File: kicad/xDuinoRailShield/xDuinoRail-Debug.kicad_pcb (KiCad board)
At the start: 2 copper layers, 99.7 x 99.7 mm, 68 parts, among them J201 USB_B, J202 SWCLK, J203 SWDIO, J204 RUN, J301 21mtc_mrkl, J401 Conn_01x06, J601 Screw_Terminal_01x02, J701 Screw_Terminal_01x02, J801 Screw_Terminal_01x02, Q901 BC847BVN, Q902 BC847BVN, U201 RP2040, U501 LM339, Y201 X322512MSB4SI

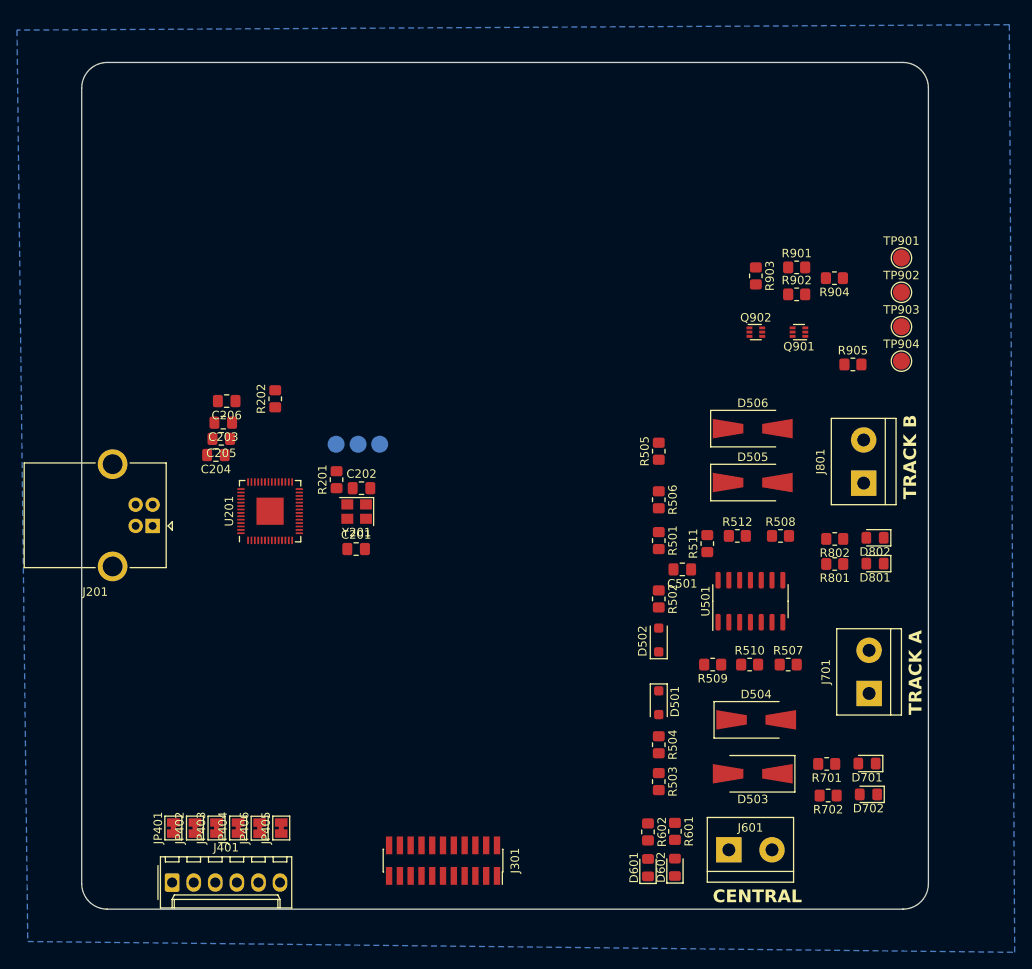
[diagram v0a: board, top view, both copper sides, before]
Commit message: More stuff
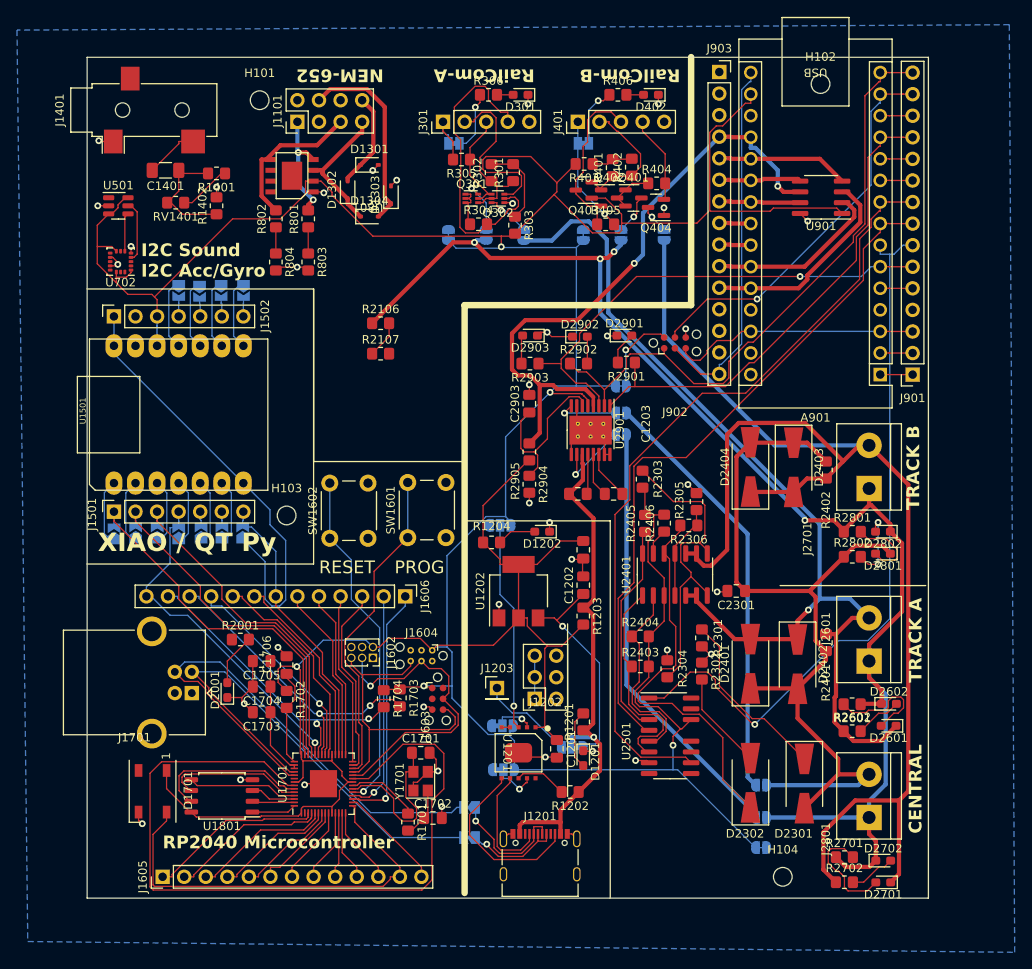
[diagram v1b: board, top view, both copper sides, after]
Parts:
- removed C201, C202: 33p, Capacitor_SMD:C_0805_2012Metric_Pad1.18x1.45mm_HandSolder
- removed C203, C204: 100n, Capacitor_SMD:C_0805_2012Metric_Pad1.18x1.45mm_HandSolder
- removed C205, C206: 10u, Capacitor_SMD:C_0805_2012Metric_Pad1.18x1.45mm_HandSolder
- removed C501: 47uF, Capacitor_SMD:C_0805_2012Metric_Pad1.18x1.45mm_HandSolder
- removed D501, D502: 1N4004, Diode_SMD:D_SOD-123F
- removed D503, D504, D505, D506: SS54, Diode_SMD:D_SMA-SMB_Universal_Handsoldering
- removed D601, D602, D701, D702, D801, D802: LED, LED_SMD:LED_0805_2012Metric_Pad1.15x1.40mm_HandSolder
- removed J202: SWCLK, TestPoint:TestPoint_Pad_D2.0mm
- removed J203: SWDIO, TestPoint:TestPoint_Pad_D2.0mm
- removed J204: RUN, TestPoint:TestPoint_Pad_D2.0mm
- removed J601, J701, J801: Screw_Terminal_01x02, TerminalBlock:TerminalBlock_bornier-2_P5.08mm
- removed JP402, JP403, JP404, JP405, JP406: SolderJumper_2_Bridged, Jumper:SolderJumper-2_P1.3mm_Bridged_Pad1.0x1.5mm
- removed Q901, Q902: BC847BVN, Package_TO_SOT_SMD:SOT-563
- removed R201: 1k, Resistor_SMD:R_0805_2012Metric_Pad1.20x1.40mm_HandSolder
- removed R202: 200R, Resistor_SMD:R_0805_2012Metric_Pad1.20x1.40mm_HandSolder
- removed R501, R502: 220R, Resistor_SMD:R_0805_2012Metric_Pad1.20x1.40mm_HandSolder
- removed R503: 270K, Resistor_SMD:R_0805_2012Metric_Pad1.20x1.40mm_HandSolder
- removed R504: 1K, Resistor_SMD:R_0805_2012Metric_Pad1.20x1.40mm_HandSolder
- removed R505: 820R, Resistor_SMD:R_0805_2012Metric_Pad1.20x1.40mm_HandSolder
- removed R506: 33k, Resistor_SMD:R_0805_2012Metric_Pad1.20x1.40mm_HandSolder
- removed R507, R508: 1R8, Resistor_SMD:R_0805_2012Metric_Pad1.20x1.40mm_HandSolder
- removed R509, R510, R511, R512: 10K, Resistor_SMD:R_0805_2012Metric_Pad1.20x1.40mm_HandSolder
- removed R601, R602, R701, R702: 3k3, Resistor_SMD:R_0805_2012Metric_Pad1.20x1.40mm_HandSolder
- removed R901, R902, R903: 10R, Resistor_SMD:R_0805_2012Metric_Pad1.20x1.40mm_HandSolder
- removed R904, R905: 10k, Resistor_SMD:R_0805_2012Metric_Pad1.20x1.40mm_HandSolder
- removed TP901, TP902, TP903, TP904: TestPoint, TestPoint:TestPoint_Pad_D2.0mm
- removed U201: RP2040, Package_DFN_QFN:QFN-56-1EP_7x7mm_P0.4mm_EP3.2x3.2mm
- removed Y201: X322512MSB4SI, Crystal:Crystal_SMD_3225-4Pin_3.2x2.5mm
- added A901: Arduino_Nano_Every, Module:Arduino_Nano, F.Cu at (177.2, 72.9)
- added C1201: 1uF, Capacitor_SMD:C_0805_2012Metric_Pad1.18x1.45mm_HandSolder, F.Cu at (139.1, 117.0)
- added C1202: 1uF, Capacitor_SMD:C_0805_2012Metric_Pad1.18x1.45mm_HandSolder, F.Cu at (142.2, 97.7)
- added C1203: 47uF, Capacitor_SMD:C_0805_2012Metric_Pad1.18x1.45mm_HandSolder, F.Cu at (142.2, 93.6)
- added C1401: 100uF, Capacitor_SMD:C_1206_3216Metric_Pad1.33x1.80mm_HandSolder, F.Cu at (93.1, 48.9)
- added C1701: 33p, Capacitor_SMD:C_0805_2012Metric_Pad1.18x1.45mm_HandSolder, F.Cu at (123.1, 117.5)
- added C1702: 33p, Capacitor_SMD:C_0805_2012Metric_Pad1.18x1.45mm_HandSolder, F.Cu at (124.5, 125.2)
- added C1703: 100n, Capacitor_SMD:C_0805_2012Metric_Pad1.18x1.45mm_HandSolder, F.Cu at (104.4, 112.7)
- added C1704: 100n, Capacitor_SMD:C_0805_2012Metric_Pad1.18x1.45mm_HandSolder, F.Cu at (104.4, 109.7)
- added C1705: 10u, Capacitor_SMD:C_0805_2012Metric_Pad1.18x1.45mm_HandSolder, F.Cu at (104.4, 106.7)
- added C1706: 10u, Capacitor_SMD:C_0805_2012Metric_Pad1.18x1.45mm_HandSolder, F.Cu at (107.3, 107.2)
- added C2301: 47uF, Capacitor_SMD:C_0805_2012Metric_Pad1.18x1.45mm_HandSolder, F.Cu at (160.3, 98.4)
- added C2901: 100nF, Capacitor_SMD:C_0805_2012Metric_Pad1.18x1.45mm_HandSolder, F.Cu at (141.6, 87.0)
- added C2902: 22nF, Capacitor_SMD:C_0805_2012Metric_Pad1.18x1.45mm_HandSolder, F.Cu at (145.8, 87.0)
- added C2903: 22nF, Capacitor_SMD:C_0805_2012Metric_Pad1.18x1.45mm_HandSolder, F.Cu at (135.9, 76.4)
- added D1201: LED, LED_SMD:LED_0603_1608Metric_Pad1.05x0.95mm_HandSolder, F.Cu at (142.2, 118.1)
- added D1202: LED, LED_SMD:LED_0603_1608Metric_Pad1.05x0.95mm_HandSolder, F.Cu at (137.4, 91.4)
- added D1301: 1N5819WS, Diode_SMD:D_SOD-323, F.Cu at (117.1, 48.3)
- added D1302: 1N5819WS, Diode_SMD:D_SOD-323, F.Cu at (114.5, 51.2)
- added D1303: 1N5819WS, Diode_SMD:D_SOD-323, F.Cu at (119.6, 51.8)
- added D1304: 1N5819WS, Diode_SMD:D_SOD-323, F.Cu at (117.1, 54.3)
- added D1701: WS2812B, LED_SMD:LED_WS2812B_PLCC4_5.0x5.0mm_P3.2mm, F.Cu at (91.5, 122.0)
- added D2001: LED, LED_SMD:LED_0603_1608Metric_Pad1.05x0.95mm_HandSolder, F.Cu at (100.3, 110.1)
- added D2301: SM4007, Diode_SMD:D_SMA-SMB_Universal_Handsoldering, F.Cu at (168.3, 121.1)
- added D2302: SM4007, Diode_SMD:D_SMA-SMB_Universal_Handsoldering, F.Cu at (161.9, 121.0)
- added D2401: SS54, Diode_SMD:D_SMA-SMB_Universal_Handsoldering, F.Cu at (161.9, 107.0)
- added D2402: SS54, Diode_SMD:D_SMA-SMB_Universal_Handsoldering, F.Cu at (167.5, 107.0)
- added D2403: SS54, Diode_SMD:D_SMA-SMB_Universal_Handsoldering, F.Cu at (167.0, 83.9)
- added D2404: SS54, Diode_SMD:D_SMA-SMB_Universal_Handsoldering, F.Cu at (161.9, 83.8)
- added D2601: LED, LED_SMD:LED_0603_1608Metric_Pad1.05x0.95mm_HandSolder, F.Cu at (178.2, 114.3)
- added D2602: LED, LED_SMD:LED_0603_1608Metric_Pad1.05x0.95mm_HandSolder, F.Cu at (178.2, 111.7)
- added D2701: LED, LED_SMD:LED_0603_1608Metric_Pad1.05x0.95mm_HandSolder, F.Cu at (177.6, 132.7)
- added D2702: LED, LED_SMD:LED_0603_1608Metric_Pad1.05x0.95mm_HandSolder, F.Cu at (177.6, 130.2)
- added D2801: LED, LED_SMD:LED_0603_1608Metric_Pad1.05x0.95mm_HandSolder, F.Cu at (177.5, 94.0)
- added D2802: LED, LED_SMD:LED_0603_1608Metric_Pad1.05x0.95mm_HandSolder, F.Cu at (177.5, 91.4)
- added D2901: LED_RED, LED_SMD:LED_0603_1608Metric_Pad1.05x0.95mm_HandSolder, F.Cu at (147.1, 68.3)
- added D2902: LED_YELLOW, LED_SMD:LED_0603_1608Metric_Pad1.05x0.95mm_HandSolder, F.Cu at (141.8, 68.5)
- added D2903: LED_GREEN, LED_SMD:LED_0603_1608Metric_Pad1.05x0.95mm_HandSolder, F.Cu at (136.0, 68.3)
- added D301: LED, LED_SMD:LED_0603_1608Metric_Pad1.05x0.95mm_HandSolder, F.Cu at (134.9, 40.0)
- added D402: LED, LED_SMD:LED_0603_1608Metric_Pad1.05x0.95mm_HandSolder, F.Cu at (150.2, 40.0)
- added H101: MountingHole, MountingHole:MountingHole_2.2mm_M2, F.Cu at (104.1, 40.6)
- added H102: MountingHole, MountingHole:MountingHole_2.2mm_M2, F.Cu at (170.2, 38.7)
- added H103: MountingHole, MountingHole:MountingHole_2.2mm_M2, F.Cu at (107.3, 89.5)
- added H104: MountingHole, MountingHole:MountingHole_2.2mm_M2, F.Cu at (165.7, 132.1)
- added J1101: Conn_02x04_Counter_Clockwise, Connector_PinHeader_2.54mm:PinHeader_2x04_P2.54mm_Vertical, F.Cu at (108.6, 43.2)
- added J1201: USB_C_Receptacle_USB2.0_14P, Connector_USB:USB_C_Receptacle_Palconn_UTC16-G, F.Cu at (137.2, 129.5)
- added J1202: Conn_02x03_Odd_Even, Connector_PinSocket_2.54mm:PinSocket_2x03_P2.54mm_Vertical, F.Cu at (136.5, 111.1)
- added J1203: Conn_01x01, Connector_PinHeader_2.54mm:PinHeader_1x01_P2.54mm_Vertical, F.Cu at (132.1, 109.9)
- added J1401: AudioJack2_Ground, Connector_Audio:Jack_3.5mm_CUI_SJ-3523-SMT_Horizontal, F.Cu at (90.5, 41.8)
- added J1501: Conn_01x07, Connector_PinSocket_2.54mm:PinSocket_1x07_P2.54mm_Vertical, F.Cu at (87.0, 89.1)
- added J1502: Conn_01x07, Connector_PinSocket_2.54mm:PinSocket_1x07_P2.54mm_Vertical, F.Cu at (87.0, 66.1)
- added J1602: Conn_02x03_Odd_Even, Connector_PinSocket_1.27mm:PinSocket_2x03_P1.27mm_Vertical, F.Cu at (117.5, 106.3)
- added J1603: Conn_ARM_SWD_TagConnect_TC2030-NL, Connector:Tag-Connect_TC2030-IDC-NL_2x03_P1.27mm_Vertical, F.Cu at (125.1, 111.1)
- added J1604: Conn_ARM_SWD_TagConnect_TC2030-NL, xDuinoRailShield:Tag-Connect_TC2030-IDC-NL_2x03_P1.27mm_Vertical-WithHoles, F.Cu at (123.2, 106.0)
- added J1605: Conn_01x13, Connector_PinHeader_2.54mm:PinHeader_1x13_P2.54mm_Vertical, F.Cu at (92.7, 132.1)
- added J1606: Conn_01x13, Connector_PinHeader_2.54mm:PinHeader_1x13_P2.54mm_Vertical, F.Cu at (121.3, 99.1)
- added J2601: Screw_Terminal_01x02, TerminalBlock:TerminalBlock_bornier-2_P5.08mm, F.Cu at (175.9, 106.7)
- added J2701: Screw_Terminal_01x02, TerminalBlock:TerminalBlock_bornier-2_P5.08mm, F.Cu at (175.9, 86.4)
- added J2801: Screw_Terminal_01x02, TerminalBlock:TerminalBlock_bornier-2_P5.08mm, F.Cu at (175.9, 125.1)
- added J901: Conn_01x15, Connector_PinSocket_2.54mm:PinSocket_1x15_P2.54mm_Vertical, F.Cu at (181.0, 73.0)
- added J902: Conn_ARM_SWD_TagConnect_TC2030-NL, Connector:Tag-Connect_TC2030-IDC-NL_2x03_P1.27mm_Vertical, F.Cu at (153.0, 69.2)
- added J903: Conn_01x15, Connector_PinSocket_2.54mm:PinSocket_1x15_P2.54mm_Vertical, F.Cu at (158.3, 37.3)
- added JP1001: SolderJumper_2_Open, Jumper:SolderJumper-2_P1.3mm_Open_RoundedPad1.0x1.5mm, B.Cu at (146.7, 77.5)
- added JP1002: SolderJumper_2_Open, Jumper:SolderJumper-2_P1.3mm_Open_RoundedPad1.0x1.5mm, B.Cu at (146.7, 80.0)
- added JP1003: SolderJumper_2_Open, Jumper:SolderJumper-2_P1.3mm_Open_RoundedPad1.0x1.5mm, B.Cu at (146.7, 74.3)
- added JP1201: CFG2, Jumper:SolderJumper-3_P1.3mm_Bridged12_RoundedPad1.0x1.5mm_NumberLabels, B.Cu at (132.7, 114.3)
- added JP1202: CFG3, Jumper:SolderJumper-3_P1.3mm_Bridged12_RoundedPad1.0x1.5mm_NumberLabels, B.Cu at (132.4, 90.7)
- added JP1203: CFG1, Jumper:SolderJumper-3_P1.3mm_Bridged12_RoundedPad1.0x1.5mm_NumberLabels, B.Cu at (132.8, 119.5)
- added JP1204: CFG1, Jumper:SolderJumper-3_P1.3mm_Bridged12_RoundedPad1.0x1.5mm_NumberLabels, B.Cu at (140.9, 116.8)
- added JP1205: SolderJumper_2_Open, Jumper:SolderJumper-2_P1.3mm_Open_TrianglePad1.0x1.5mm, B.Cu at (128.8, 123.9)
- added JP1206: SolderJumper_2_Open, Jumper:SolderJumper-2_P1.3mm_Open_TrianglePad1.0x1.5mm, B.Cu at (128.8, 127.5)
- added JP1501: SolderJumper_2_Open, Jumper:SolderJumper-2_P1.3mm_Open_TrianglePad1.0x1.5mm, B.Cu at (87.0, 91.7)
- added JP1502: SolderJumper_2_Open, Jumper:SolderJumper-2_P1.3mm_Open_TrianglePad1.0x1.5mm, B.Cu at (92.1, 91.6)
- added JP1503: SolderJumper_2_Open, Jumper:SolderJumper-2_P1.3mm_Open_TrianglePad1.0x1.5mm, B.Cu at (89.5, 91.6)
- added JP1504: SolderJumper_2_Open, Jumper:SolderJumper-2_P1.3mm_Open_TrianglePad1.0x1.5mm, B.Cu at (94.6, 91.7)
- added JP1505: SolderJumper_2_Open, Jumper:SolderJumper-2_P1.3mm_Open_TrianglePad1.0x1.5mm, B.Cu at (97.2, 91.6)
- added JP1506: SolderJumper_2_Open, Jumper:SolderJumper-2_P1.3mm_Open_TrianglePad1.0x1.5mm, B.Cu at (99.7, 91.6)
- added JP1507: SolderJumper_2_Open, Jumper:SolderJumper-2_P1.3mm_Open_TrianglePad1.0x1.5mm, B.Cu at (102.1, 91.6)
- added JP1508: SolderJumper_2_Open, Jumper:SolderJumper-2_P1.3mm_Open_TrianglePad1.0x1.5mm, B.Cu at (102.2, 63.0)
- added JP1509: SolderJumper_2_Open, Jumper:SolderJumper-2_P1.3mm_Open_TrianglePad1.0x1.5mm, B.Cu at (99.6, 63.0)
- added JP1510: SolderJumper_2_Open, Jumper:SolderJumper-2_P1.3mm_Open_TrianglePad1.0x1.5mm, B.Cu at (97.1, 63.1)
- added JP1511: SolderJumper_2_Open, Jumper:SolderJumper-2_P1.3mm_Open_TrianglePad1.0x1.5mm, B.Cu at (94.6, 63.0)
- added JP1901: SolderJumper_2_Open, Jumper:SolderJumper-2_P1.3mm_Open_RoundedPad1.0x1.5mm, B.Cu at (135.3, 56.5)
- added JP1902: SolderJumper_2_Open, Jumper:SolderJumper-2_P1.3mm_Open_RoundedPad1.0x1.5mm, B.Cu at (130.8, 56.5)
- added JP1903: SolderJumper_2_Open, Jumper:SolderJumper-2_P1.3mm_Open_RoundedPad1.0x1.5mm, B.Cu at (126.4, 56.5)
- added JP201: SolderJumper_2_Open, Jumper:SolderJumper-2_P1.3mm_Open_RoundedPad1.0x1.5mm, B.Cu at (151.8, 56.5)
- added JP202: SolderJumper_2_Open, Jumper:SolderJumper-2_P1.3mm_Open_RoundedPad1.0x1.5mm, B.Cu at (146.7, 56.5)
- added JP203: SolderJumper_2_Open, Jumper:SolderJumper-2_P1.3mm_Open_RoundedPad1.0x1.5mm, B.Cu at (142.2, 56.5)
- added JP301: SolderJumper_2_Bridged, Jumper:SolderJumper-2_P1.3mm_Bridged_Pad1.0x1.5mm, B.Cu at (127.0, 45.7)
- added JP601: SolderJumper_2_Open, Jumper:SolderJumper-2_P1.3mm_Open_RoundedPad1.0x1.5mm, B.Cu at (163.2, 121.3)
- added JP602: SolderJumper_2_Open, Jumper:SolderJumper-2_P1.3mm_Open_RoundedPad1.0x1.5mm, B.Cu at (163.2, 125.1)
- added JP603: SolderJumper_2_Open, Jumper:SolderJumper-2_P1.3mm_Open_RoundedPad1.0x1.5mm, B.Cu at (163.2, 128.6)
- added Q301: BC847BVN, Package_TO_SOT_SMD:SOT-563, F.Cu at (129.1, 52.2)
- added Q302: BC847BVN, Package_TO_SOT_SMD:SOT-563, F.Cu at (132.2, 52.2)
- added Q401: S8050, Package_TO_SOT_SMD:SOT-23, F.Cu at (148.1, 52.2)
- added Q402: S8550, Package_TO_SOT_SMD:SOT-23, F.Cu at (145.3, 52.2)
- added Q403: S8550, Package_TO_SOT_SMD:SOT-23, F.Cu at (142.3, 51.2)
- added Q404: S8050, Package_TO_SOT_SMD:SOT-23, F.Cu at (150.8, 53.3)
- added R1201: 1k, Resistor_SMD:R_0805_2012Metric_Pad1.20x1.40mm_HandSolder, F.Cu at (142.2, 113.8)
- added R1202: 10k, Resistor_SMD:R_0805_2012Metric_Pad1.20x1.40mm_HandSolder, F.Cu at (140.7, 122.1)
- added R1203: 1k, Resistor_SMD:R_0805_2012Metric_Pad1.20x1.40mm_HandSolder, F.Cu at (142.2, 101.4)
- added R1204: 100R, Resistor_SMD:R_0805_2012Metric_Pad1.20x1.40mm_HandSolder, F.Cu at (131.4, 92.7)
- added R1401: 10k, Resistor_SMD:R_0805_2012Metric_Pad1.20x1.40mm_HandSolder, F.Cu at (99.1, 49.3)
- added R1402: 10k, Resistor_SMD:R_0805_2012Metric_Pad1.20x1.40mm_HandSolder, F.Cu at (99.1, 53.1)
- added R1701: 1k, Resistor_SMD:R_0805_2012Metric_Pad1.20x1.40mm_HandSolder, F.Cu at (121.6, 125.6)
- added R1702: 220R, Resistor_SMD:R_0805_2012Metric_Pad1.20x1.40mm_HandSolder, F.Cu at (107.3, 111.2)
- added R1703: 10k, Resistor_SMD:R_0805_2012Metric_Pad1.20x1.40mm_HandSolder, F.Cu at (120.7, 111.0)
- added R1704: 10k, Resistor_SMD:R_0805_2012Metric_Pad1.20x1.40mm_HandSolder, F.Cu at (118.7, 111.1)
- added R2001: 470R, Resistor_SMD:R_0805_2012Metric_Pad1.20x1.40mm_HandSolder, F.Cu at (101.9, 104.1)
- added R2106: 10k, Resistor_SMD:R_0805_2012Metric_Pad1.20x1.40mm_HandSolder, F.Cu at (118.4, 66.9)
- added R2107: 10k, Resistor_SMD:R_0805_2012Metric_Pad1.20x1.40mm_HandSolder, F.Cu at (118.4, 70.5)
- added R2301: 220R, Resistor_SMD:R_0805_2012Metric_Pad1.20x1.40mm_HandSolder, F.Cu at (156.2, 104.0)
- added R2302: 220R, Resistor_SMD:R_0805_2012Metric_Pad1.20x1.40mm_HandSolder, F.Cu at (156.2, 107.9)
- added R2303: 180K, Resistor_SMD:R_0805_2012Metric_Pad1.20x1.40mm_HandSolder, F.Cu at (149.2, 85.3)
- added R2304: 1k, Resistor_SMD:R_0805_2012Metric_Pad1.20x1.40mm_HandSolder, F.Cu at (152.1, 107.6)
- added R2305: 820R, Resistor_SMD:R_0805_2012Metric_Pad1.20x1.40mm_HandSolder, F.Cu at (155.6, 87.9)
- added R2306: 33k, Resistor_SMD:R_0805_2012Metric_Pad1.20x1.40mm_HandSolder, F.Cu at (154.7, 90.7)
- added R2401: 1R8, Resistor_SMD:R_0805_2012Metric_Pad1.20x1.40mm_HandSolder, F.Cu at (170.8, 104.5)
- added R2402: 1R8, Resistor_SMD:R_0805_2012Metric_Pad1.20x1.40mm_HandSolder, F.Cu at (170.8, 84.2)
- added R2403: 10k, Resistor_SMD:R_0805_2012Metric_Pad1.20x1.40mm_HandSolder, F.Cu at (149.0, 107.3)
- added R2404: 10k, Resistor_SMD:R_0805_2012Metric_Pad1.20x1.40mm_HandSolder, F.Cu at (149.0, 103.8)
- added R2405: 10k, Resistor_SMD:R_0805_2012Metric_Pad1.20x1.40mm_HandSolder, F.Cu at (149.5, 90.5)
- added R2406: 10k, Resistor_SMD:R_0805_2012Metric_Pad1.20x1.40mm_HandSolder, F.Cu at (151.8, 90.4)
- added R2601: 3k3, Resistor_SMD:R_0805_2012Metric_Pad1.20x1.40mm_HandSolder, F.Cu at (173.9, 111.8)
- added R2602: 3k3, Resistor_SMD:R_0805_2012Metric_Pad1.20x1.40mm_HandSolder, F.Cu at (173.9, 114.9)
- added R2701: 3k3, Resistor_SMD:R_0805_2012Metric_Pad1.20x1.40mm_HandSolder, F.Cu at (173.0, 129.8)
- added R2702: 3k3, Resistor_SMD:R_0805_2012Metric_Pad1.20x1.40mm_HandSolder, F.Cu at (173.0, 132.7)
- added R2801: 3k3, Resistor_SMD:R_0805_2012Metric_Pad1.20x1.40mm_HandSolder, F.Cu at (173.9, 91.5)
- added R2802: 3k3, Resistor_SMD:R_0805_2012Metric_Pad1.20x1.40mm_HandSolder, F.Cu at (173.9, 94.4)
- added R2901: 470R, Resistor_SMD:R_0805_2012Metric_Pad1.20x1.40mm_HandSolder, F.Cu at (147.3, 71.5)
- added R2902: 470R, Resistor_SMD:R_0805_2012Metric_Pad1.20x1.40mm_HandSolder, F.Cu at (141.7, 71.7)
- added R2903: 470R, Resistor_SMD:R_0805_2012Metric_Pad1.20x1.40mm_HandSolder, F.Cu at (136.0, 71.7)
- added R2904: 1k5, Resistor_SMD:R_0805_2012Metric_Pad1.20x1.40mm_HandSolder, F.Cu at (135.9, 85.9)
- added R2905: 47k, Resistor_SMD:R_0805_2012Metric_Pad1.20x1.40mm_HandSolder, F.Cu at (135.9, 82.0)
- added R301: 10R, Resistor_SMD:R_0805_2012Metric_Pad1.20x1.40mm_HandSolder, F.Cu at (134.0, 49.2)
- added R302: 10R, Resistor_SMD:R_0805_2012Metric_Pad1.20x1.40mm_HandSolder, F.Cu at (131.4, 49.2)
- added R303: 10R, Resistor_SMD:R_0805_2012Metric_Pad1.20x1.40mm_HandSolder, F.Cu at (134.2, 55.4)
- added R304: 10k, Resistor_SMD:R_0805_2012Metric_Pad1.20x1.40mm_HandSolder, F.Cu at (129.9, 55.2)
- added R305: 10k, Resistor_SMD:R_0805_2012Metric_Pad1.20x1.40mm_HandSolder, F.Cu at (127.9, 47.6)
- added R306: 100R, Resistor_SMD:R_0805_2012Metric_Pad1.20x1.40mm_HandSolder, F.Cu at (131.1, 40.0)
- added R401: 10R, Resistor_SMD:R_0805_2012Metric_Pad1.20x1.40mm_HandSolder, F.Cu at (145.7, 48.6)
- added R402: 10R, Resistor_SMD:R_0805_2012Metric_Pad1.20x1.40mm_HandSolder, F.Cu at (148.0, 48.5)
- added R403: 10R, Resistor_SMD:R_0805_2012Metric_Pad1.20x1.40mm_HandSolder, F.Cu at (142.3, 48.1)
- added R404: 10k, Resistor_SMD:R_0805_2012Metric_Pad1.20x1.40mm_HandSolder, F.Cu at (150.9, 50.4)
- added R405: 10k, Resistor_SMD:R_0805_2012Metric_Pad1.20x1.40mm_HandSolder, F.Cu at (144.9, 55.3)
- added R406: 100R, Resistor_SMD:R_0805_2012Metric_Pad1.20x1.40mm_HandSolder, F.Cu at (146.3, 40.0)
- added R803: 1k, Resistor_SMD:R_0805_2012Metric_Pad1.20x1.40mm_HandSolder, F.Cu at (109.9, 59.7)
- added R804: 1k, Resistor_SMD:R_0805_2012Metric_Pad1.20x1.40mm_HandSolder, F.Cu at (106.0, 59.7)
- added RV1401: 10k, Resistor_SMD:R_0805_2012Metric_Pad1.20x1.40mm_HandSolder, F.Cu at (94.2, 52.7)
- added SW1601: SW_Push, Button_Switch_THT:SW_PUSH_6mm, F.Cu at (121.6, 92.2)
- added SW1602: SW_Push, Button_Switch_THT:SW_PUSH_6mm, F.Cu at (112.4, 92.2)
- added U1201: ~, Debug-Shield-Lib:CH224K, F.Cu at (134.6, 117.5)
- added U1202: AMS1117-3.3, Package_TO_SOT_SMD:SOT-223-3_TabPin2, F.Cu at (134.6, 98.5)
- added U1501: MOUDLE-SEEEDUINO-XIAO-ESP32C3, xiao ESP32C3_PCB:MOUDLE14P-SMD-2.54-21X17.8MM, F.Cu at (105.1, 86.6)
- added U1701: RP2040, Package_DFN_QFN:QFN-56-1EP_7x7mm_P0.4mm_EP3.2x3.2mm, F.Cu at (111.7, 121.1)
- added U1801: W25Q128JVS, Package_SO:SOIC-8_5.23x5.23mm_P1.27mm, F.Cu at (99.7, 122.6)
- added U2401: LM339, Package_SO:SOIC-14_3.9x8.7mm_P1.27mm, F.Cu at (153.0, 96.5)
- added U2501: 74HC02, Package_SO:SOIC-14-16_3.9x9.9mm_P1.27mm, F.Cu at (152.5, 115.5)
- added U2901: DRV8874PWPR, Package_SO:HTSSOP-16-1EP_4.4x5mm_P0.65mm_EP3.4x5mm_Mask2.46x2.31mm_ThermalVias, F.Cu at (143.1, 79.5)
- added U702: LIS3DH, Package_LGA:LGA-16_3x3mm_P0.5mm_LayoutBorder3x5y, F.Cu at (87.8, 59.6)
- added U801: BDR6133, BDR6133:BDR6133, F.Cu at (108.0, 49.5)
- added U901: ATtiny402-SS, Package_SO:SOIC-8_3.9x4.9mm_P1.27mm, F.Cu at (170.2, 52.1)
- added Y1701: X322512MSB4SI, Crystal:Crystal_SMD_3225-4Pin_3.2x2.5mm, F.Cu at (123.1, 120.8)
- J301: value 21mtc_mrkl -> Conn_01x05; footprint Connector_PinSocket_1.27mm:PinSocket_2x11_P1.27mm_Vertical_SMD -> Connector_PinHeader_2.54mm:PinHeader_1x05_P2.54mm_Vertical
- J401: value Conn_01x06 -> Conn_01x05; footprint Connector_Molex:Molex_KK-254_AE-6410-06A_1x06_P2.54mm_Vertical -> Connector_PinHeader_2.54mm:PinHeader_1x05_P2.54mm_Vertical
- JP401: moved to B.Cu
- R801, R802: value 3k3 -> 6k8
- U501: value LM339 -> MCP4725xxx-xCH; footprint Package_SO:SOIC-14_3.9x8.7mm_P1.27mm -> Package_TO_SOT_SMD:SOT-23-6
- moved J401 101.5 mm to (141.6, 43.2), turned to 90 degrees
- moved JP401 94.0 mm to (142.3, 45.7), turned to 180 degrees
- moved U501 87.8 mm to (87.5, 53.1), turned to 0 degrees
- moved J301 87.0 mm to (125.7, 43.2), turned to 90 degrees
- moved R802 75.8 mm to (106.0, 54.6), turned to 90 degrees
- moved R801 74.1 mm to (109.9, 54.6), turned to 90 degrees
- moved J1701 20.2 mm to (96.2, 110.5)
- renumbered J201 to J1701
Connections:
- net /loco-adapter-nem651-6-pin/AMP_MOTOR1 renamed /rails_signal_feedback_dcc-railcom-8x50/RAILCOM_DATA
- J1701 pad 2: Net-(J201-D-) -> /USB_DM
- J1701 pad 3: Net-(J201-D+) -> /USB_DP
- J301 pad 1: /loco-adapter-maerklin-21mtc/AUX7 -> /rails_signal_feedback_dcc-railcom_BC8x7/RAILCOM_DATA
- J301 pad 2: /loco-adapter-maerklin-21mtc/DCC1 -> /rails_signal_feedback_dcc-railcom_BC8x7/RC_CURR
- J301 pad 3: /loco-adapter-maerklin-21mtc/AUX8 -> /rails_signal_feedback_dcc-railcom_BC8x7/RC_FB_IN
- J301 pad 4: /loco-adapter-maerklin-21mtc/DCC0 -> /rails_signal_feedback_dcc-railcom_BC8x7/RC_ON_OFF
- J301 pad 5: /loco-adapter-maerklin-21mtc/AUX6 -> GND
- J401 pad 2: /loco-adapter-nem651-6-pin/AMP_MOTOR0 -> /rails_signal_feedback_dcc-railcom-8x50/RC_CURR
- J401 pad 3: /loco-adapter-nem651-6-pin/DCC1 -> /rails_signal_feedback_dcc-railcom-8x50/RC_FB_IN
- J401 pad 4: /loco-adapter-nem651-6-pin/DCC0 -> /rails_signal_feedback_dcc-railcom-8x50/RC_ON_OFF
- J401 pad 5: /loco-adapter-nem651-6-pin/FUNC1 -> GND
- JP401 pad 1: unconnected-(JP401-A-Pad1) -> Net-(JP401-A)
- R801 pad 1: /TRACK_B1 -> /ADC0
- R801 pad 2: Net-(D801-A) -> /AMP_MOTOR0
- R802 pad 1: /TRACK_B0 -> /ADC1
- R802 pad 2: Net-(D802-A) -> /AMP_MOTOR1
- U501 pad 1: /central_railcom-detector/RAILCOM_A1 -> /i2c-audio-ic/SPEAKER1
- U501 pad 2: /central_railcom-detector/RAILCOM_A0 -> GND
- U501 pad 3: +5V -> +3V3
- U501 pad 4: -18mv -> /GPIO24
- U501 pad 5: /TRACK_A0 -> /GPIO25
- U501 pad 6: /TRACK_A0 -> +3V3
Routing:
- net +3V3: track 0.00 -> 523.5 mm, vias 0 -> 6
- net /TRACK_B0: track 0.00 -> 164.3 mm
- net /CENTRAL_MAIN1: track 0.00 -> 161.7 mm, vias 0 -> 4
- net /TRACK_A0: track 0.00 -> 117.8 mm, vias 0 -> 1
- net /CENTRAL_MAIN0: track 0.00 -> 101.3 mm
- net Net-(U1701-DVDD-Pad23): track 0.00 -> 94.3 mm
- net /CN_D6: track 0.00 -> 92.6 mm
- net /CN_D4: track 0.00 -> 86.0 mm, vias 0 -> 1
- net GND: track 0.00 -> 85.4 mm, vias 0 -> 37
- net /CN_D5: track 0.00 -> 81.1 mm
- net /CN_A0: track 0.00 -> 74.5 mm, vias 0 -> 2
- net /CN_D12: track 0.00 -> 74.3 mm
- net /USB_DP: track 0.00 -> 61.4 mm
- net +VBUS_H: track 0.00 -> 60.7 mm, vias 0 -> 1
- net /CN_D9: track 0.00 -> 58.5 mm
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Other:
- board size 99.7 x 99.7 mm -> 99.1 x 99 mm
- board text added: "I2C Sound I2C Acc/Gyro"
- board text added: "NEM-652"
- board text added: "PROG"
- board text added: "RESET"
- board text added: "RP2040 Microcontroller"
- board text added: "RailCom-A"
- board text added: "RailCom-B"
- board text added: "XIAO / QT Py"
